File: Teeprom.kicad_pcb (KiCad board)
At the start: 2 copper layers, 16 x 38 mm, 4 parts, among them J1 Tandy_100_102_200_option_rom, U1 28C256

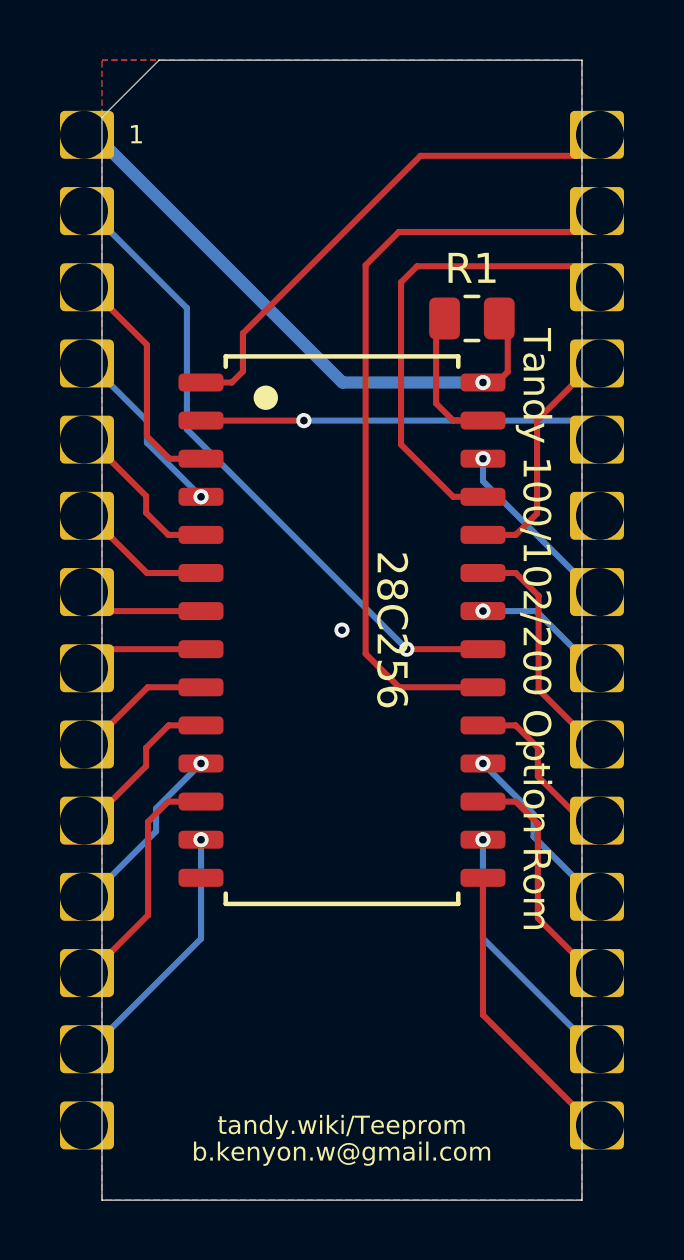
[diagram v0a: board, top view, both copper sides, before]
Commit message: cosmetics
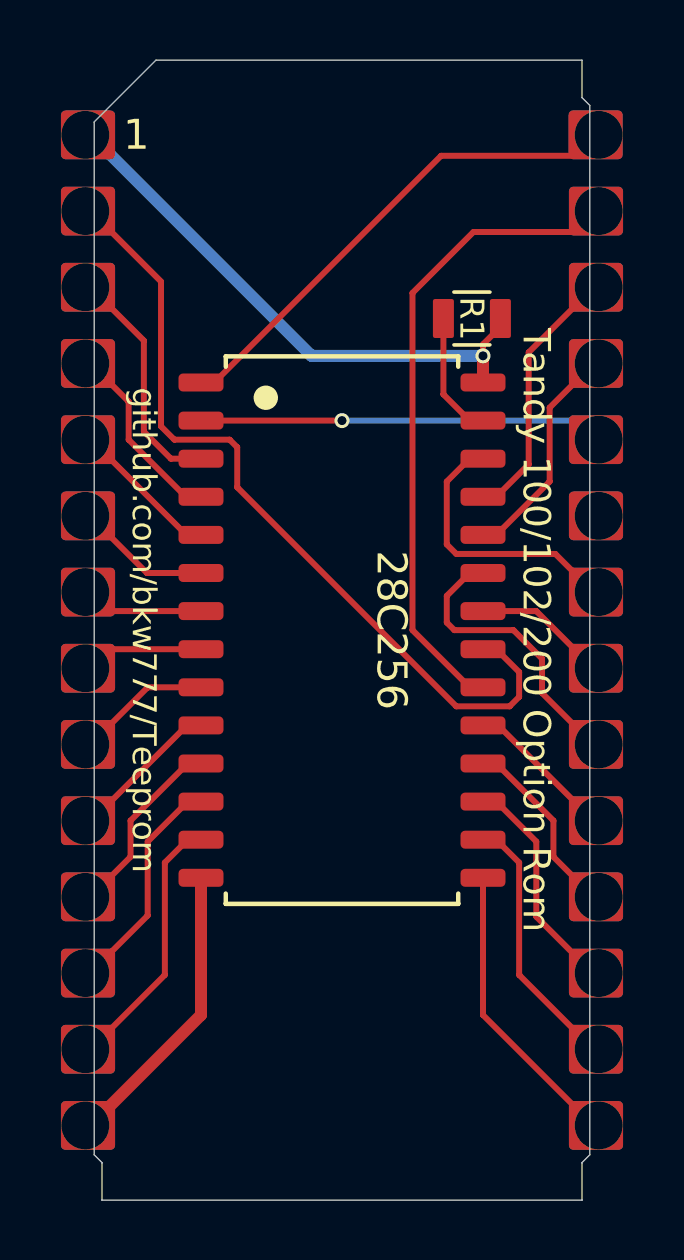
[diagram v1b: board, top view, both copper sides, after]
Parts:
- removed carrier?: pcb2molex8878_chamfer, 000_LOCAL:pcb2molex8878_chamfer
- J1: footprint 000_LOCAL:pcb2molex8878 -> 000_LOCAL:Molex78805_PCB
- R1: footprint 000_LOCAL:R_0805_2012Metric -> 000_LOCAL:R_0805
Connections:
- net /VCC renamed VCC
- net /VSS renamed GND
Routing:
- net GND: track 0.00 -> 9.95 mm, vias 1 -> 0
- net /A8: track 15.9 -> 8.89 mm
- net /A10: track 21.6 -> 27.5 mm, vias 1 -> 0
- net /~CE: track 25.9 -> 21.7 mm
- net /A13: track 6.09 -> 9.34 mm, vias 1 -> 0
- net /A11: track 8.01 -> 9.78 mm
- net VCC: track 19.6 -> 18.7 mm
- net /A14: track 17.4 -> 16.6 mm
- net /D7: track 5.69 -> 5.12 mm
- net /~WE: track 4.73 -> 4.17 mm
- net /A6: track 6.08 -> 6.54 mm, vias 1 -> 0
- net /D4: track 8.63 -> 8.94 mm, vias 1 -> 0
- net /D6: track 6.09 -> 6.40 mm, vias 1 -> 0
- net /D0: track 6.10 -> 6.40 mm, vias 1 -> 0
- net /D2: track 8.64 -> 8.94 mm, vias 1 -> 0
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- removed copper zone on B.Cu, net GND
- removed copper zone on F.Cu, net GND
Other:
- board size 16 x 38 mm -> 16.5 x 38 mm
- net class Default: clearance 0.2032 -> 0.2; trace_width 0.2032 -> 0.2; via_dia 0.508 -> 0.5; via_drill 0.254 -> 0.3
- rule trace_clearance: 0.2032 -> 0.2
- rule trace_min: 0.1524 -> 0.2
- rule via_min_drill: 0.254 -> 0.3
- rule via_min_size: 0.508 -> 0.5
- board text added: "Use with carrier: http://shpws.me/RqW3"
- board text added: "github.com/bkw777/Teeprom"
- board text removed: "Use with thingiverse.com/thing:3821586"
- board text removed: "b.kenyon.w@gmail.com"
- board text removed: "tandy.wiki/Teeprom"
